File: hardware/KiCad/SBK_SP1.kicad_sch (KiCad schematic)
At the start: 10 parts, among them J1 1x4 pin header, Q1 AO3400A, Q2 AO3401A

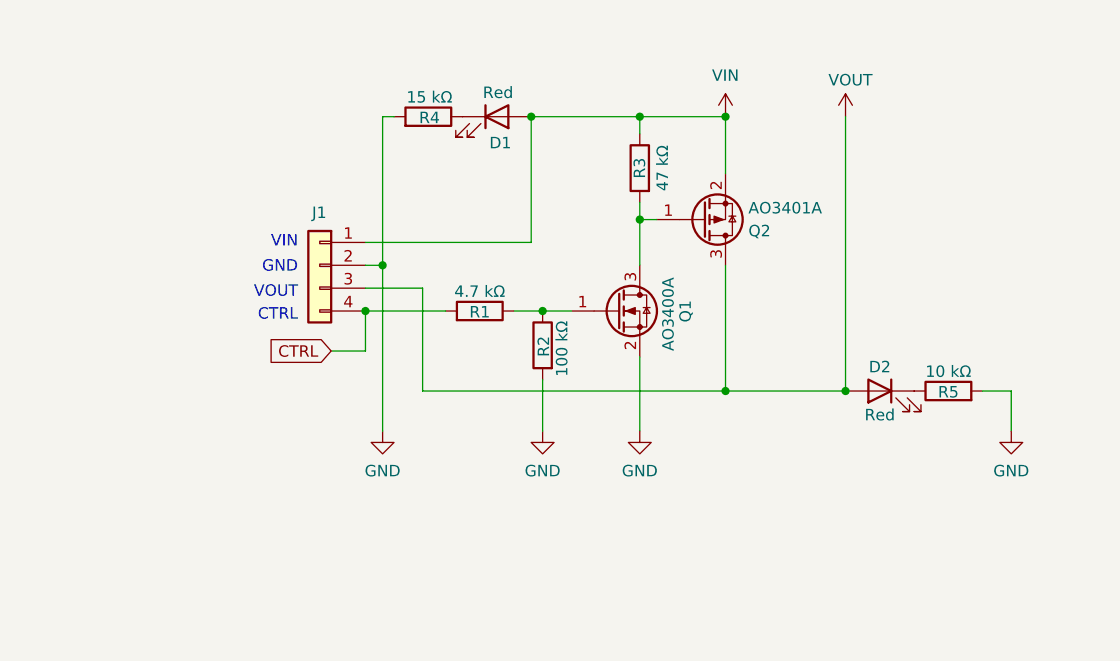
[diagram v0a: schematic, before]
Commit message: SBK_SP1 V2..0 updates
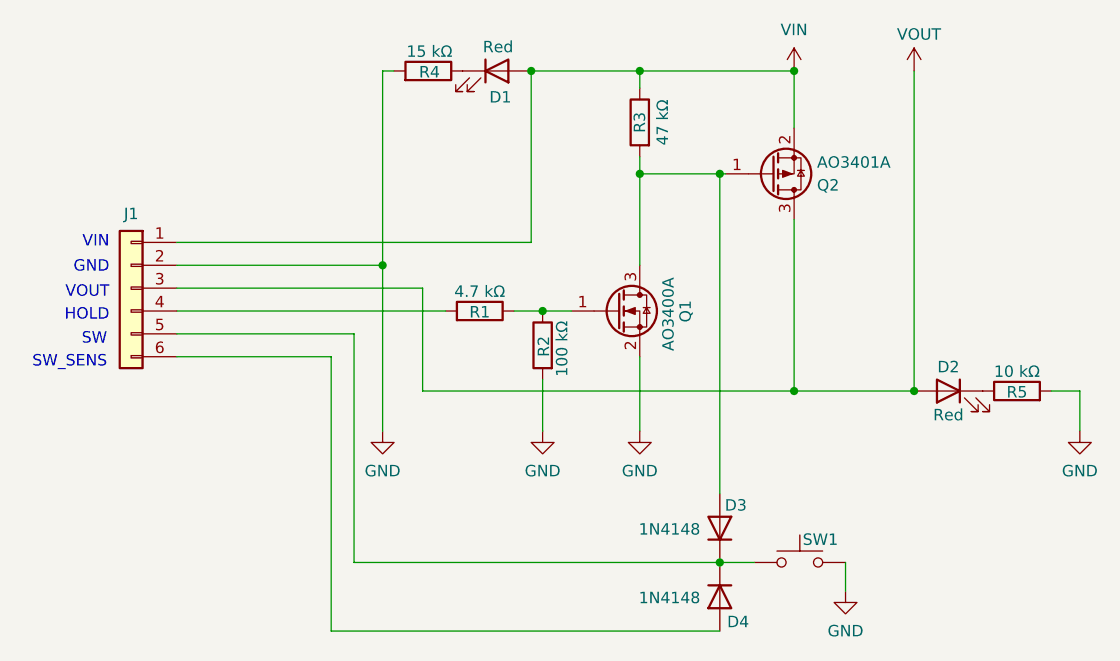
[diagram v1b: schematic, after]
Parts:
- removed J1: 1x4 pin header, Connector_PinHeader_2.54mm:PinHeader_1x04_P2.54mm_Vertical, symbol Connector_Generic:Conn_01x04
- added D3, D4: 1N4148, Diode_SMD:D_SOD-323, symbol Diode:1N4148WS
- added J1: Conn_01x06, Connector_PinHeader_2.54mm:PinHeader_1x06_P2.54mm_Vertical, symbol Connector_Generic:Conn_01x06
- added SW1: TS-1088-AR02016, Button_Switch_SMD:SW_SPST_TS-1088-xR020, symbol Switch:SW_Push
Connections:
- net GND: now also J1.2 (Pin_2), SW1.2
- net VIN: now also J1.1 (Pin_1)
- net VOUT: now also J1.3 (Pin_3)
- net at Q1.3 (D), Q2.1 (G), R3.2: now also D3.2 (A)
- net CTRL: no longer names the net of R1.2
- net CTRL: now also J1.4 (Pin_4)
- new net: D3.1 (K), D4.1 (K), J1.5 (Pin_5), SW1.1
- new net: D4.2 (A), J1.6 (Pin_6)
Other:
- note added: "HOLD"
- note added: "SW"
- note added: "SW_SENS"
- note removed: "CTRL"
- moved on the sheet: D1, D2, Q2, R3, R4, R5
